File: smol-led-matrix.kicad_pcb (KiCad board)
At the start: 4 copper layers, 20.4 x 20.4 mm, 226 parts, among them U1 STM32L431CBTx

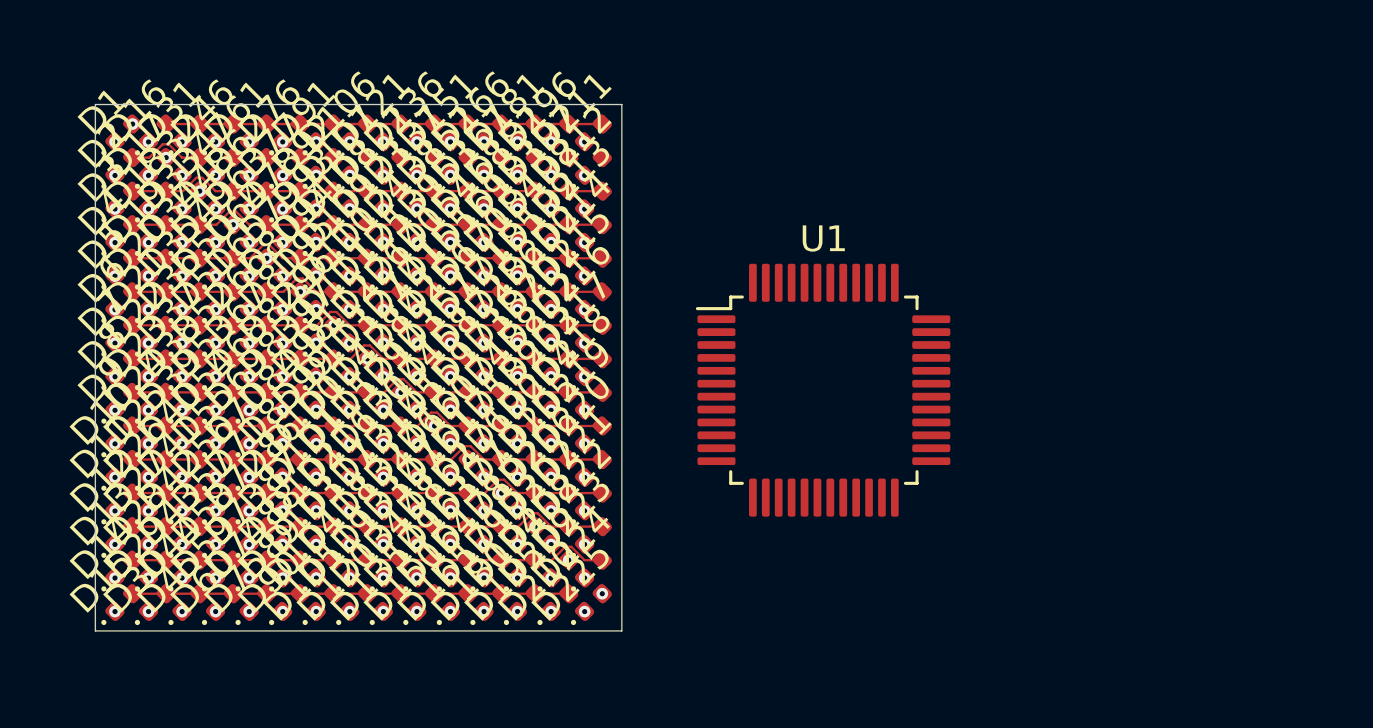
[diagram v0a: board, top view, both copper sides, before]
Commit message: Place parts
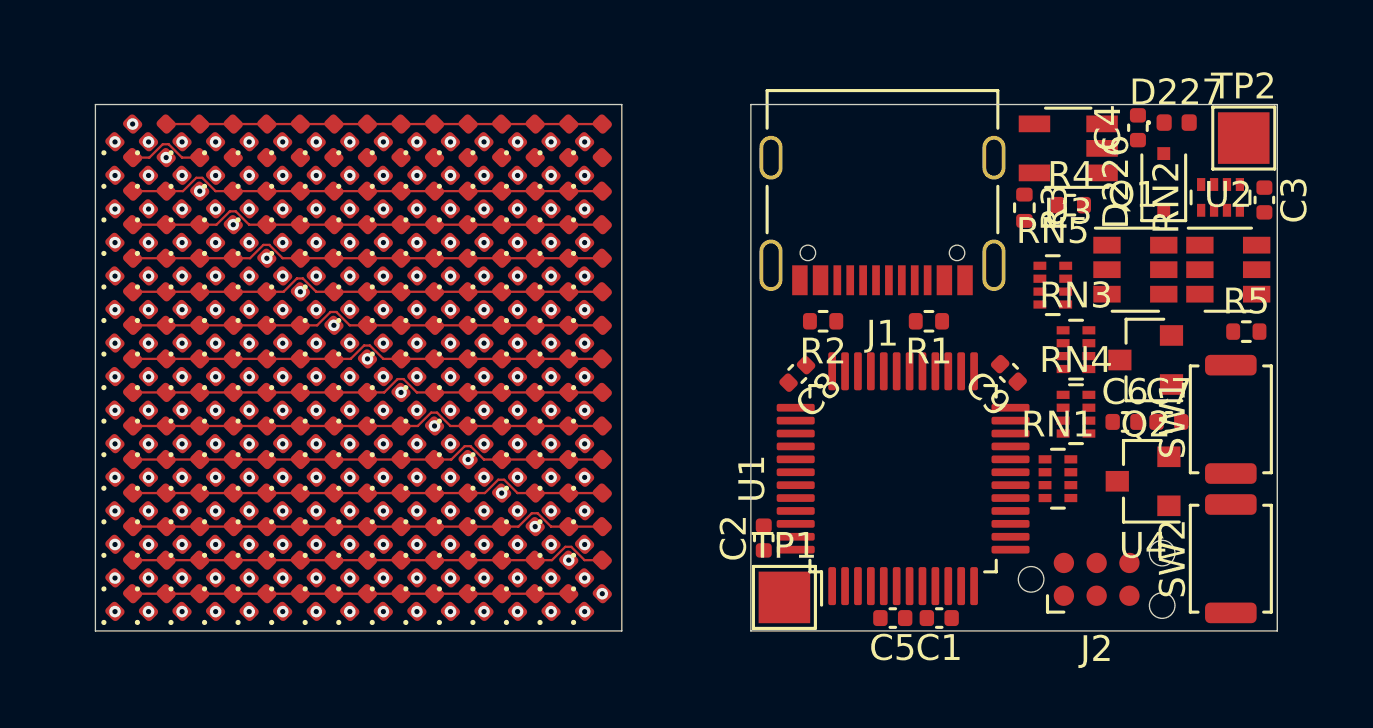
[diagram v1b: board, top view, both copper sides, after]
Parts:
- added C1: 100nF, Capacitor_SMD:C_0402_1005Metric, F.Cu at (131.6, 118.8)
- added C2: 100nF, Capacitor_SMD:C_0402_1005Metric, F.Cu at (124.8, 115.7)
- added C3: 100nF, Capacitor_SMD:C_0402_1005Metric, F.Cu at (144.2, 102.6)
- added C4: 1uF, Capacitor_SMD:C_0402_1005Metric, F.Cu at (139.3, 99.8)
- added C5: 100nF, Capacitor_SMD:C_0402_1005Metric, F.Cu at (129.8, 118.8)
- added C6: 1uF, Capacitor_SMD:C_0402_1005Metric, F.Cu at (138.8, 111.2)
- added C7: 1uF, Capacitor_SMD:C_0402_1005Metric, F.Cu at (140.5, 111.2)
- added C8: 100nF, Capacitor_SMD:C_0402_1005Metric, F.Cu at (126.1, 109.3)
- added C9: 100nF, Capacitor_SMD:C_0402_1005Metric, F.Cu at (134.3, 109.3)
- added D226: 1N4148, Diode_SMD:D_SOD-323F, F.Cu at (140.3, 101.9)
- added D227: LED, LED_SMD:LED_0402_1005Metric, F.Cu at (140.8, 99.6)
- added J1: USB_C_Receptacle_USB2.0, Connector_USB:USB_C_Receptacle_Palconn_UTC16-G, F.Cu at (129.4, 103.2)
- added J2: TagConnect_TC2030_SWD, Connector:Tag-Connect_TC2030-IDC-NL_2x03_P1.27mm_Vertical, F.Cu at (137.7, 117.3)
- added Q1: FS8205, Package_TO_SOT_SMD:SOT-23-6, F.Cu at (139.2, 105.3)
- added Q2: AO3401A, Package_TO_SOT_SMD:SOT-23, F.Cu at (139.6, 108.8)
- added R1: 5.1kR, Resistor_SMD:R_0402_1005Metric, F.Cu at (131.2, 107.3)
- added R2: 5.1kR, Resistor_SMD:R_0402_1005Metric, F.Cu at (127.1, 107.3)
- added R3: 27kR, Resistor_SMD:R_0402_1005Metric, F.Cu at (134.9, 102.9)
- added R4: 27kR, Resistor_SMD:R_0402_1005Metric, F.Cu at (136.7, 102.8)
- added R5: 27kR, Resistor_SMD:R_0402_1005Metric, F.Cu at (143.5, 107.7)
- added RN1: 1kR, Resistor_SMD:R_Array_Concave_4x0402, F.Cu at (136.2, 113.4)
- added RN2: 1kR, Resistor_SMD:R_Array_Concave_4x0402, F.Cu at (142.5, 102.5)
- added RN3: 1kR, Resistor_SMD:R_Array_Concave_4x0402, F.Cu at (136.9, 108.4)
- added RN4: 1kR, Resistor_SMD:R_Array_Concave_4x0402, F.Cu at (136.9, 110.9)
- added RN5: 1kR, Resistor_SMD:R_Array_Concave_4x0402, F.Cu at (136.0, 105.9)
- added SW1: SW_Push, Button_Switch_SMD:SW_Push_SPST_NO_Alps_SKRK, F.Cu at (142.9, 111.1)
- added SW2: SW_Push, Button_Switch_SMD:SW_Push_SPST_NO_Alps_SKRK, F.Cu at (142.9, 116.5)
- added TP1: BAT+, TestPoint:TestPoint_Pad_2.0x2.0mm, F.Cu at (125.6, 118.0)
- added TP2: BAT-, TestPoint:TestPoint_Pad_2.0x2.0mm, F.Cu at (143.4, 100.2)
- added U2: DW01+G, Package_TO_SOT_SMD:SOT-23-6, F.Cu at (142.8, 105.3)
- added U3: TP4054, Package_TO_SOT_SMD:TSOT-23-5, F.Cu at (136.6, 100.6)
- added U4: XC6206P332MR, Package_TO_SOT_SMD:SOT-23, F.Cu at (139.5, 113.5)
- U1: value STM32L431CBTx -> STM32L433CBTx
- moved U1 4.60 mm to (130.2, 113.4), turned to 90 degrees
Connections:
- net Net-(U1-Pad28) renamed /K15
- U1 pad 18: Net-(U1-Pad18) -> /K0
- U1 pad 19: Net-(U1-Pad19) -> /K1
- U1 pad 20: Net-(U1-Pad20) -> /K2
- U1 pad 21: Net-(U1-Pad21) -> /K10
- U1 pad 22: Net-(U1-Pad22) -> /K11
- U1 pad 23: Net-(U1-Pad23) -> GND
- U1 pad 24: Net-(U1-Pad24) -> +3V3
- U1 pad 25: Net-(U1-Pad25) -> /K12
- U1 pad 26: Net-(U1-Pad26) -> /K13
- U1 pad 27: Net-(U1-Pad27) -> /K14
- U1 pad 32: Net-(U1-Pad32) -> /D-
- U1 pad 33: Net-(U1-Pad33) -> /D+
- U1 pad 35: Net-(U1-Pad35) -> GND
- U1 pad 36: Net-(U1-Pad36) -> +3V3
- U1 pad 39: Net-(U1-Pad39) -> /K3
- U1 pad 40: Net-(U1-Pad40) -> /K4
- U1 pad 41: Net-(U1-Pad41) -> /K5
- U1 pad 42: Net-(U1-Pad42) -> /K6
- U1 pad 43: Net-(U1-Pad43) -> /K7
- U1 pad 45: Net-(U1-Pad45) -> /K8
- U1 pad 46: Net-(U1-Pad46) -> /K9
- U1 pad 47: Net-(U1-Pad47) -> GND
- U1 pad 48: Net-(U1-Pad48) -> +3V3
- U1 pad 7: Net-(U1-Pad7) -> /~RST
- U1 pad 8: Net-(U1-Pad8) -> GND
- U1 pad 9: Net-(U1-Pad9) -> +3V3
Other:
- board size 20.4 x 20.4 mm -> 45.8 x 20.4 mm
